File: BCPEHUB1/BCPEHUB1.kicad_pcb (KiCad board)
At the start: 2 copper layers, 31 parts, among them J1 Conn_01x02_Female, J10 Conn_01x05_Female, J4 Conn_01x02_Female, U1 TP4056, U2 DW01, U3 FS8205A, U4 ESP32-WROOM-32D, U5 BMP180, U6 HTU21DSMD

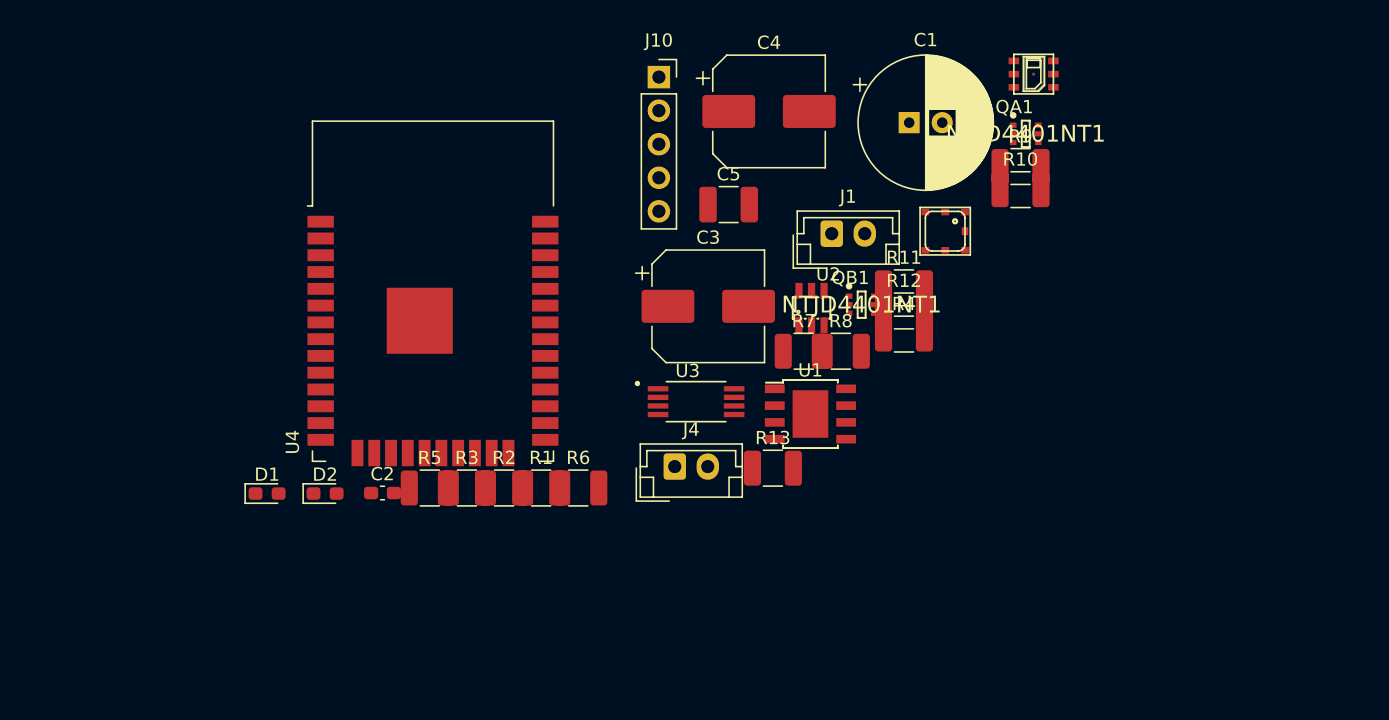
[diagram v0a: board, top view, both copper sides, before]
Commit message: Add files via upload
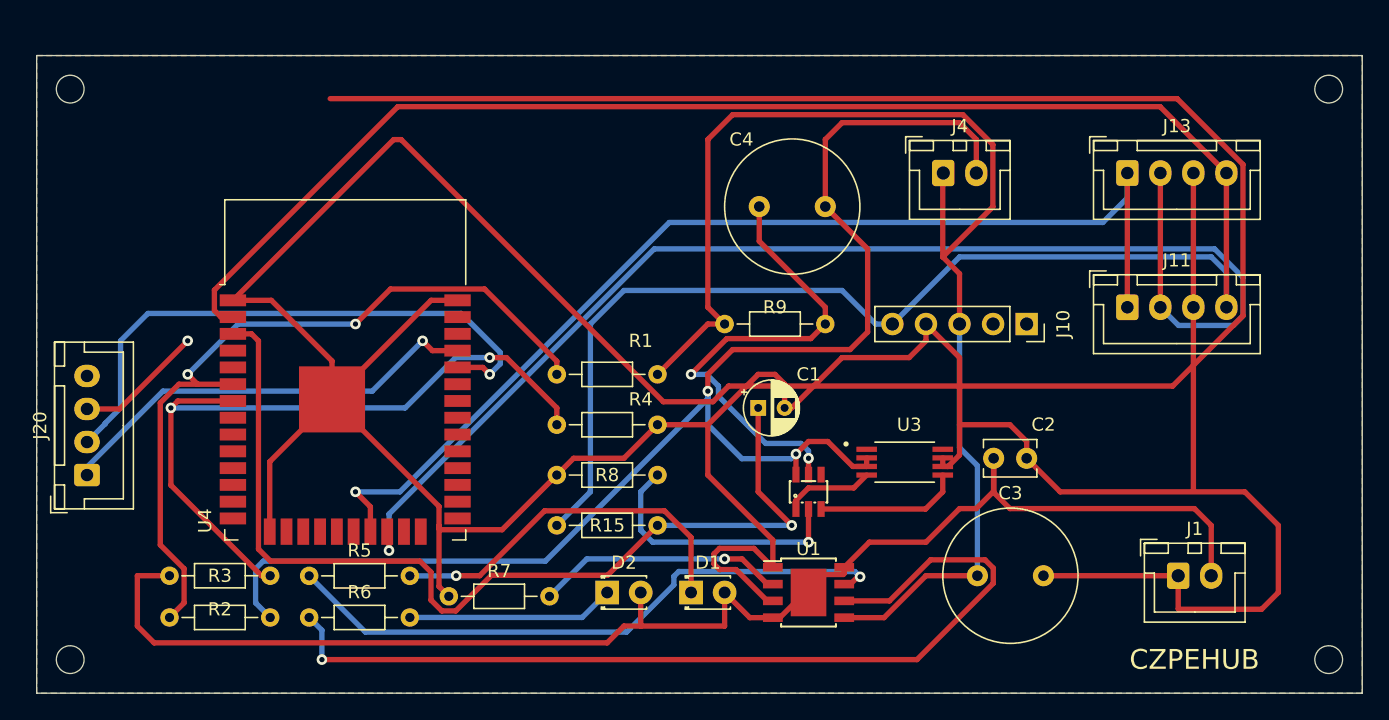
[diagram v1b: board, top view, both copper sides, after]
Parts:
- removed C5: 100n, Capacitor_SMD:C_1210_3225Metric_Pad1.33x2.70mm_HandSolder
- removed QA1, QB1: NTJD4401NT1, eec:On_Semiconductor-NTJD4401NT1-Manufacturer_Recommended
- removed R10, R11, R12, R13: 10k, Resistor_SMD:R_1210_3225Metric_Pad1.30x2.65mm_HandSolder
- removed U5: BMP180, SparkFun-Sensors:BMP180
- removed U6: HTU21DSMD, SparkFun-Sensors:HTU21D
- added J11: Conn_01x04_Female, Connector_JST:JST_XH_B4B-XH-A_1x04_P2.50mm_Vertical, F.Cu at (180.3, 94.0)
- added J13: Conn_01x04_Female, Connector_JST:JST_XH_B4B-XH-A_1x04_P2.50mm_Vertical, F.Cu at (180.3, 83.8)
- added J20: Conn_01x03_Female, Connector_JST:JST_XH_B4B-XH-A_1x04_P2.50mm_Vertical, F.Cu at (101.6, 106.7)
- added R15: 10k, Resistor_THT:R_Axial_DIN0204_L3.6mm_D1.6mm_P7.62mm_Horizontal, F.Cu at (137.2, 110.5)
- added REF**: MountingHole_2.1mm, MountingHole:MountingHole_2.1mm, F.Cu at (100.3, 77.5)
- added REF**: MountingHole_2.1mm, MountingHole:MountingHole_2.1mm, F.Cu at (100.3, 120.7)
- added REF**: MountingHole_2.1mm, MountingHole:MountingHole_2.1mm, F.Cu at (195.6, 120.7)
- added REF**: MountingHole_2.1mm, MountingHole:MountingHole_2.1mm, F.Cu at (195.6, 77.5)
- C1: footprint Capacitor_THT:CP_Radial_D10.0mm_P2.50mm -> Capacitor_THT:CP_Radial_D4.0mm_P2.00mm
- C2: footprint Capacitor_SMD:C_0603_1608Metric_Pad1.08x0.95mm_HandSolder -> Capacitor_THT:C_Disc_D3.8mm_W2.6mm_P2.50mm
- C3, C4: footprint Capacitor_SMD:CP_Elec_8x6.5 -> Capacitor_THT:C_Radial_D10.0mm_H12.5mm_P5.00mm
- D1, D2: footprint LED_SMD:LED_0603_1608Metric_Pad1.05x0.95mm_HandSolder -> LED_THT:LED_D1.8mm_W3.3mm_H2.4mm
- J1, J4: footprint Connector_JST:JST_EH_B2B-EH-A_1x02_P2.50mm_Vertical -> Connector_JST:JST_XH_B2B-XH-A_1x02_P2.50mm_Vertical
- R1, R2, R3, R4, R5, R6, R7, R8, R9: footprint Resistor_SMD:R_1210_3225Metric_Pad1.30x2.65mm_HandSolder -> Resistor_THT:R_Axial_DIN0204_L3.6mm_D1.6mm_P7.62mm_Horizontal
- moved C2 46.3 mm to (170.2, 105.4)
- moved J1 36.9 mm to (184.2, 114.3)
- moved J10 33.5 mm to (172.7, 95.2), turned to 270 degrees
- moved D1 33.0 mm to (147.3, 115.6)
- moved R7 32.6 mm to (129.0, 115.9)
- moved J4 30.1 mm to (166.4, 83.8)
- moved C3 28.8 mm to (169.0, 114.3)
- moved R4 27.2 mm to (137.2, 102.9)
- moved R2 27.2 mm to (107.8, 117.5)
- moved R9 25.4 mm to (149.9, 95.2)
- moved C1 24.4 mm to (152.4, 101.6)
- moved R3 23.5 mm to (107.8, 114.3)
- moved R8 23.4 mm to (137.2, 106.7)
- moved D2 22.6 mm to (141.0, 115.6)
- moved R6 22.6 mm to (118.4, 117.5)
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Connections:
- net OUT+ renamed 3,3V+
- net OUT- renamed GND
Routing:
- net GND: track 0.00 -> 404.3 mm, vias 0 -> 1
- net 3,3V+: track 0.00 -> 169.5 mm
- net BAT-: track 0.00 -> 109.0 mm, vias 0 -> 2
- net SOL+: track 0.00 -> 108.6 mm
- net Net-(J11-Pad2): track 0.00 -> 98.3 mm, vias 0 -> 1
- net BAT+: track 0.00 -> 97.6 mm
- net Net-(J11-Pad1): track 0.00 -> 83.2 mm, vias 0 -> 1
- net Net-(C1-Pad1): track 0.00 -> 74.1 mm, vias 0 -> 1
- net Net-(R6-Pad1): track 0.00 -> 70.8 mm, vias 0 -> 1
- net Net-(R1-Pad2): track 0.00 -> 58.5 mm, vias 0 -> 2
- net Net-(R3-Pad2): track 0.00 -> 54.7 mm, vias 0 -> 2
- net Net-(R5-Pad1): track 0.00 -> 47.3 mm, vias 0 -> 1
- net Net-(J20-Pad2): track 0.00 -> 44.2 mm, vias 0 -> 1
- net Net-(C4-Pad1): track 0.00 -> 36.2 mm, vias 0 -> 2
- net Net-(J20-Pad1): track 0.00 -> 32.9 mm, vias 0 -> 1
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- added copper zone on B.Cu, net GND
- added copper zone on F.Cu, net GND
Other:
- board outline added: 100.3 x 48.3 mm
- rule trace_min: 0.2 -> 0.25
- board text added: "CZPEHUB"
